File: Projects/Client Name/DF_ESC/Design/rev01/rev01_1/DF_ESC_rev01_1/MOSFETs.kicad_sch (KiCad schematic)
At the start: 21 parts, among them Q1 HSBA15810C, Q2 HSBA15810C, Q3 HSBA15810C, Q4 HSBA15810C, Q5 HSBA15810C, Q6 HSBA15810C

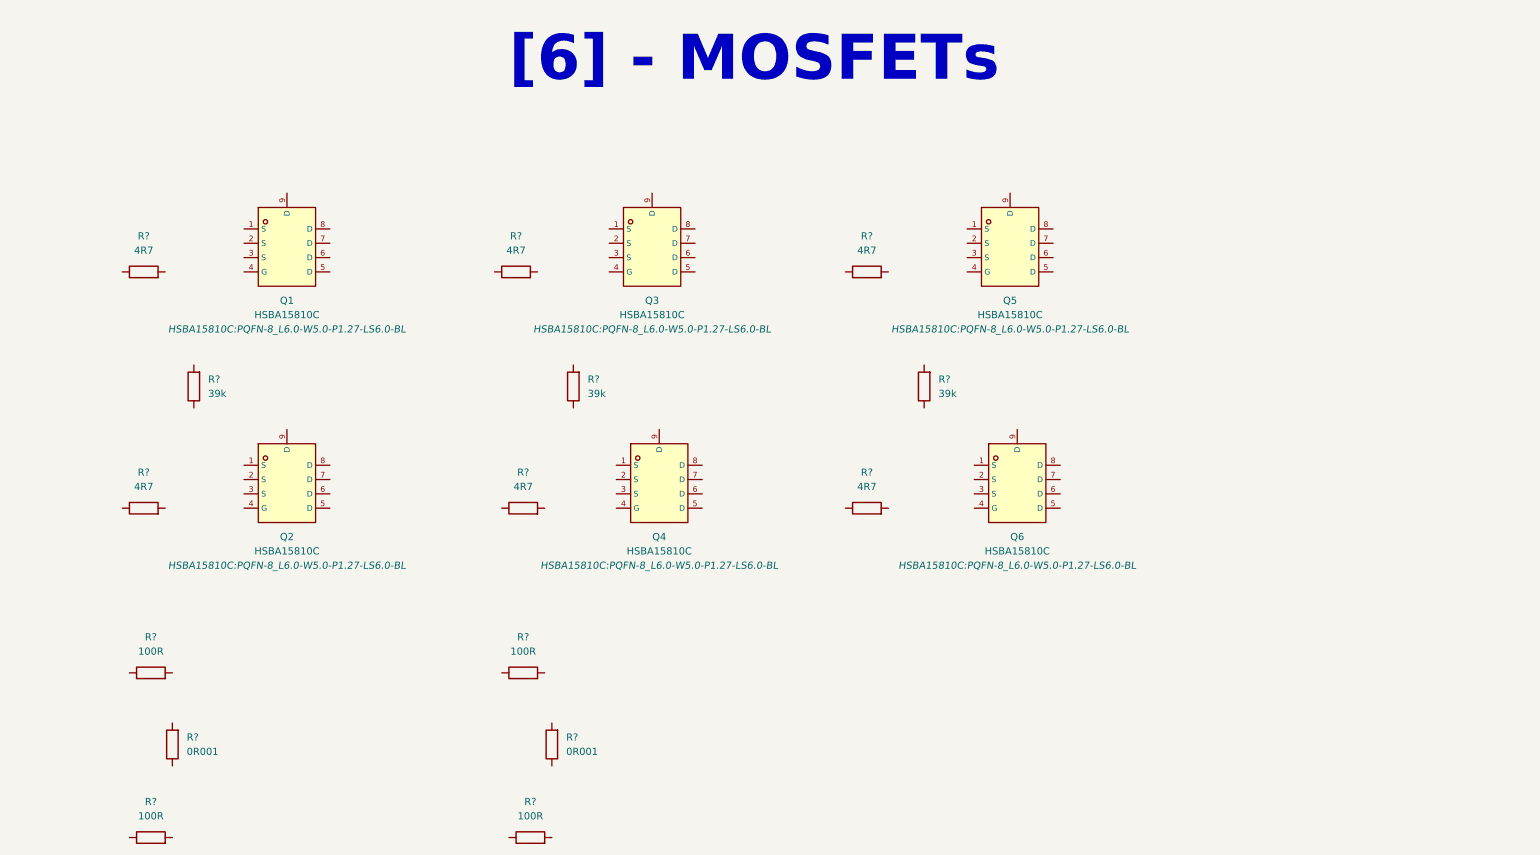
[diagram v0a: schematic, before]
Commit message: home Santander 24-02-2024
Acabados los mosfets
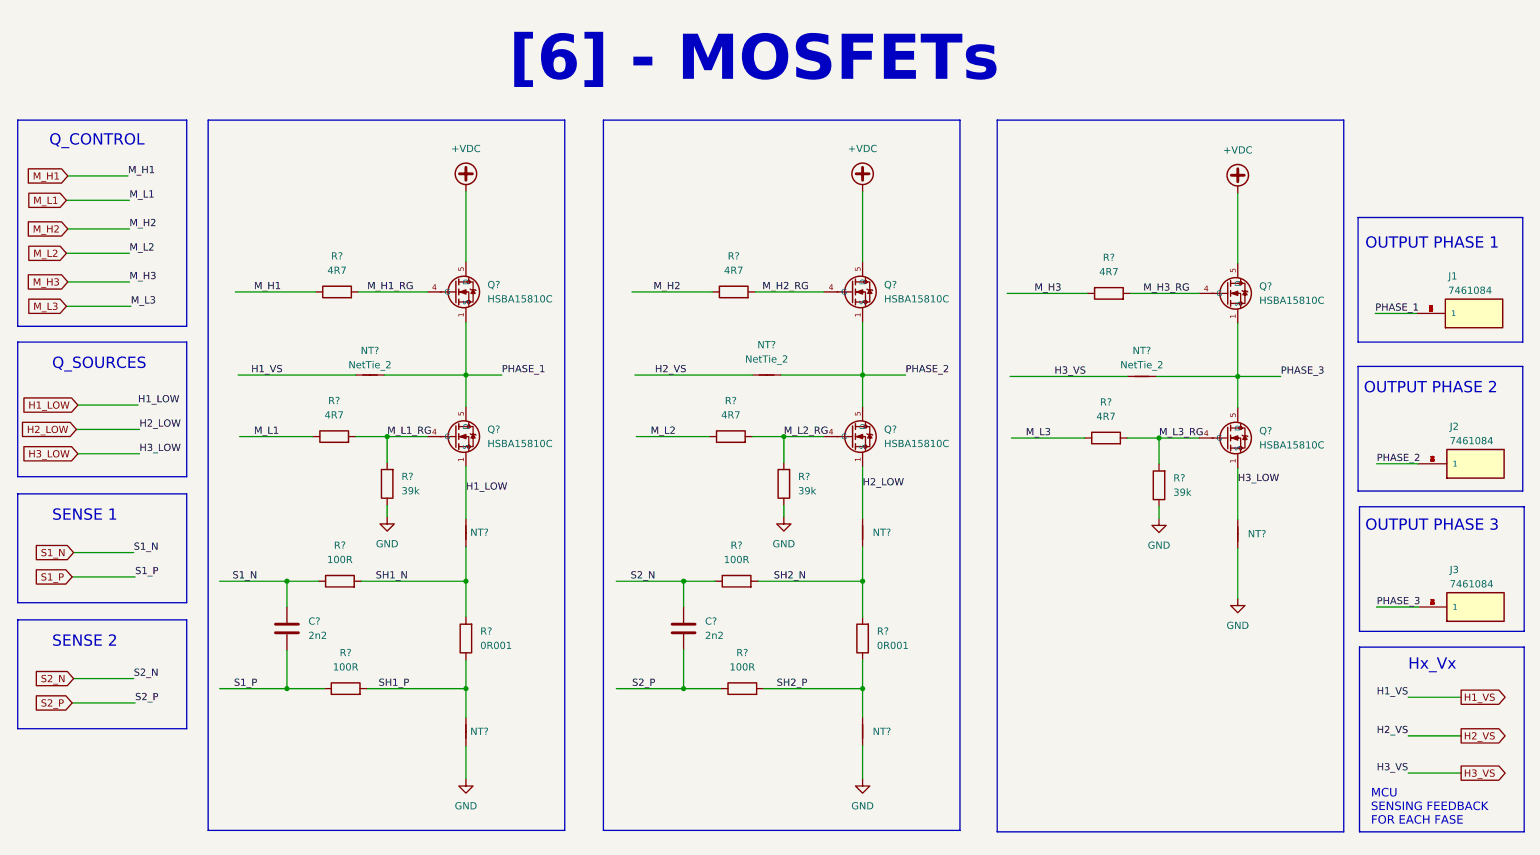
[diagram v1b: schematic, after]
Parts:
- removed Q1, Q2, Q3, Q4, Q5, Q6: HSBA15810C, HSBA15810C:PQFN-8_L6.0-W5.0-P1.27-LS6.0-BL, symbol Mosfet_HSBA15810C:HSBA15810C
- removed R? (x4): 100R, symbol Device:R
- removed R? (x3): 39k, symbol Device:R
- removed R? (x6): 4R7, symbol Device:R
- removed R? (x2): 0R001, symbol Device:R
- added C? (x2): 2n2, symbol Device:C
- added J1, J2, J3: 7461084, 7461084:WE_7461084, symbol 7461084:7461084
- added NT? (x6): NetTie_2, symbol Device:NetTie_2
- added NT? (x2): ~, symbol Device:NetTie_2
- added Q? (x6): HSBA15810C, DF_ESC_Footprint_Library:PQFN-8_L6.0-W5.0-P1.27-LS6.0-BL, symbol DF_ESC_Symbol_Library:HSBA15810C
- added R? (x6): 4R7, symbol Device:R
- added R? (x3): 39k, symbol Device:R
- added R? (x4): 100R, symbol Device:R
- added R? (x2): 0R001, symbol Device:R
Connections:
- new net +VDC: Q?.5 (D), Q?.5 (D), Q?.5 (D), Q?.6 (D), Q?.6 (D), Q?.6 (D), Q?.7 (D), Q?.7 (D), Q?.7 (D), Q?.8 (D), Q?.8 (D), Q?.8 (D), Q?.9 (D), Q?.9 (D), Q?.9 (D)
- new net GND: NT?.1, NT?.1, NT?.1, R?.1, R?.1, R?.1
- new net H1_LOW: NT?.2, Q?.1 (S), Q?.2 (S), Q?.3 (S)
- new net H1_VS: NT?.2
- new net H2_LOW: NT?.2, Q?.1 (S), Q?.2 (S), Q?.3 (S)
- new net H2_VS: NT?.2
- new net H3_LOW: NT?.2, Q?.1 (S), Q?.2 (S), Q?.3 (S)
- new net H3_VS: NT?.2
- new net M_H1: R?.1
- new net M_H1_RG: Q?.4 (G), R?.2
- new net M_H2: R?.1
- new net M_H2_RG: Q?.4 (G), R?.2
- new net M_H3: R?.1
- new net M_H3_RG: Q?.4 (G), R?.2
- new net M_L1: R?.1
- new net M_L1_RG: Q?.4 (G), R?.2, R?.2
- new net M_L2: R?.1
- new net M_L2_RG: Q?.4 (G), R?.2, R?.2
- new net M_L3: R?.1
- new net M_L3_RG: Q?.4 (G), R?.2, R?.2
- new net PHASE_1: J1.1, J1.2 (1), J1.3 (1), J1.4 (1), J1.5 (1), J1.6 (1), J1.7 (1), J1.8 (1), NT?.1, Q?.1 (S), Q?.2 (S), Q?.3 (S), Q?.5 (D), Q?.6 (D), Q?.7 (D), Q?.8 (D), Q?.9 (D)
- new net PHASE_2: J2.1, J2.2 (1), J2.3 (1), J2.4 (1), J2.5 (1), J2.6 (1), J2.7 (1), J2.8 (1), NT?.1, Q?.1 (S), Q?.2 (S), Q?.3 (S), Q?.5 (D), Q?.6 (D), Q?.7 (D), Q?.8 (D), Q?.9 (D)
- new net PHASE_3: J3.1, J3.2 (1), J3.3 (1), J3.4 (1), J3.5 (1), J3.6 (1), J3.7 (1), J3.8 (1), NT?.1, Q?.1 (S), Q?.2 (S), Q?.3 (S), Q?.5 (D), Q?.6 (D), Q?.7 (D), Q?.8 (D), Q?.9 (D)
- new net S1_N: C?.1, R?.1
- new net S1_P: C?.2, R?.1
- new net S2_N: C?.1, R?.1
- new net S2_P: C?.2, R?.1
- new net SH1_N: NT?.1, R?.2, R?.2
- new net SH1_P: NT?.2, R?.1, R?.2
- new net SH2_N: NT?.1, R?.2, R?.2
- new net SH2_P: NT?.2, R?.1, R?.2
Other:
- note added: "Hx_Vx"
- note added: "MCU SENSING FEEDBACK FOR EACH FASE"
- note added: "OUTPUT PHASE 1"
- note added: "OUTPUT PHASE 2"
- note added: "OUTPUT PHASE 3"
- note added: "Q_CONTROL"
- note added: "Q_SOURCES"
- note added: "SENSE 1"
- note added: "SENSE 2"
